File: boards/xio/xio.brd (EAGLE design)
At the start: 170 x 170 mm, 249 parts, among them CN3 J00-0065NL, U2 LAN8742A-CZ, X2 USB-A, Y1 NX3225SA-12.000MHZ-STD-CSR-1, Y2 NX3225SA-12.000MHZ-STD-CSR-1, Y3 NX3225SA-25.000MHZ-STD-CSR-1

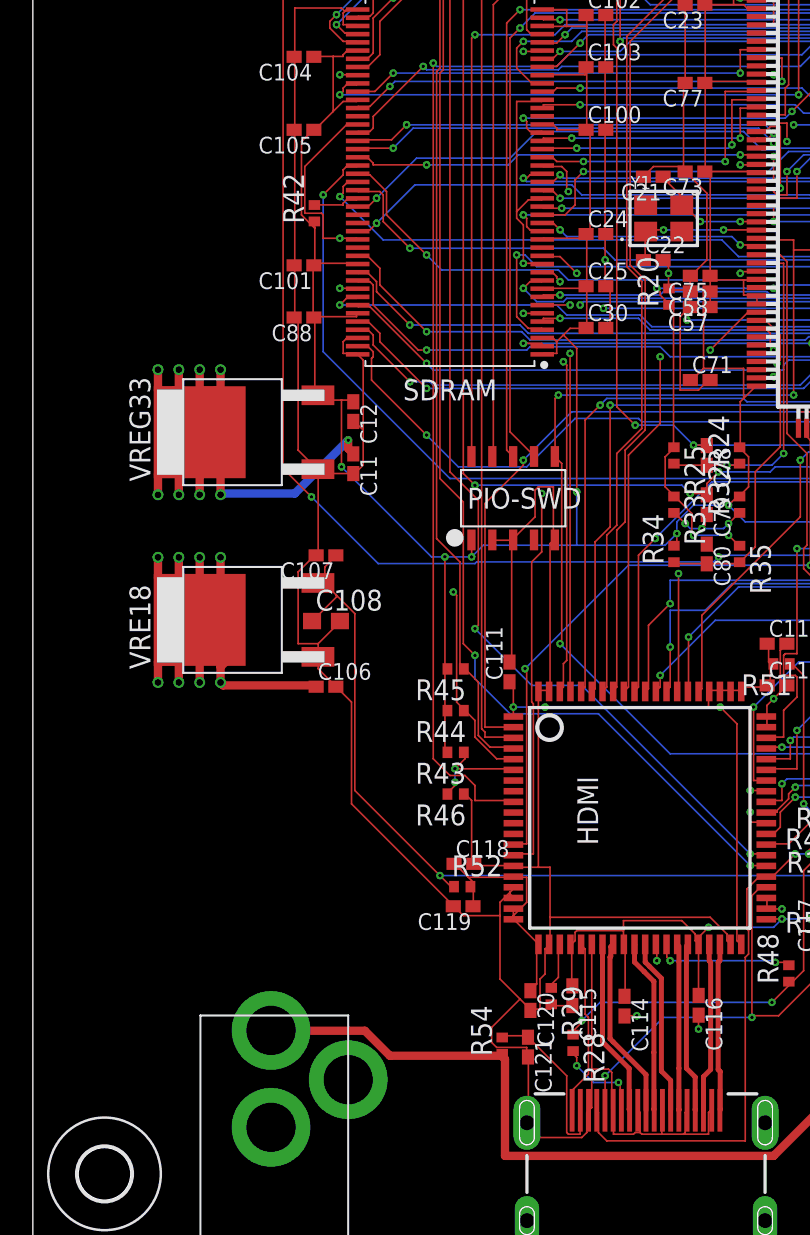
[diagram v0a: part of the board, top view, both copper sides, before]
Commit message: Last minute changes prior to review
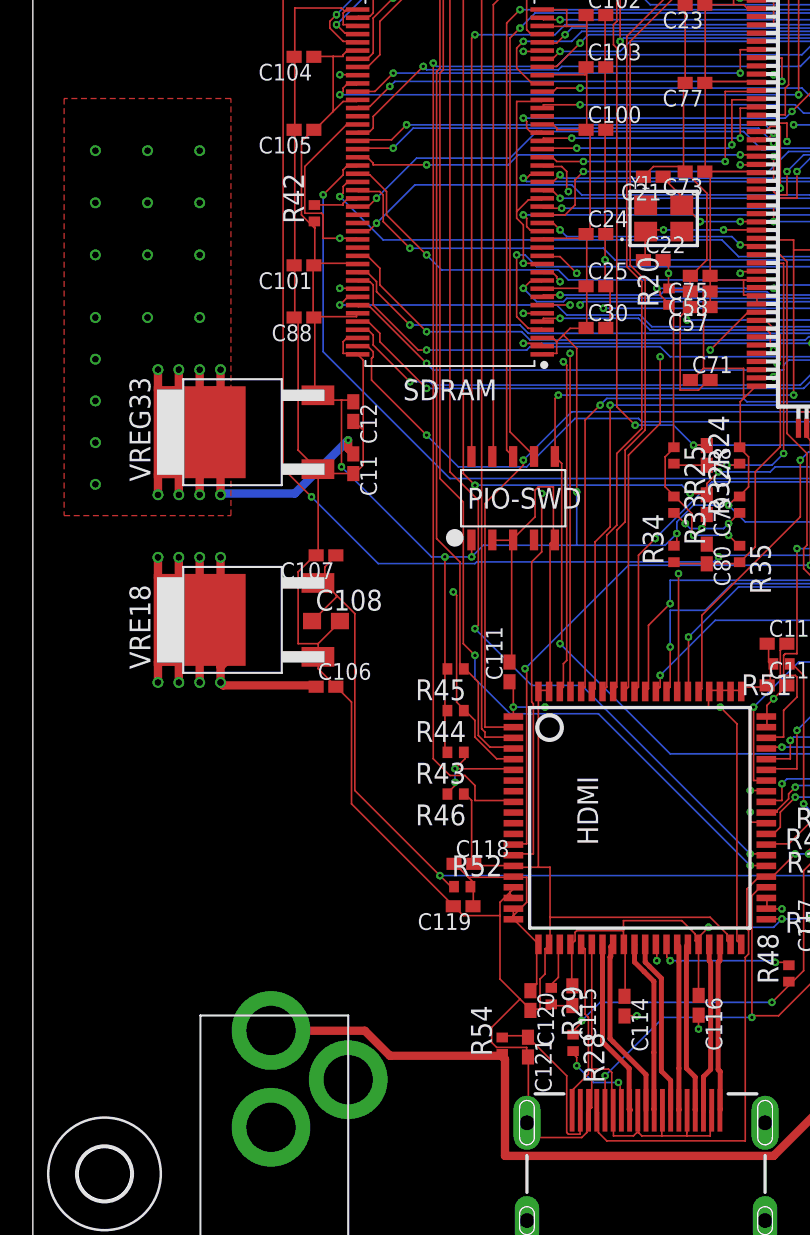
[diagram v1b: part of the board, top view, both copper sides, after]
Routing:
- net +5V: vias 76 -> 92
- added copper zone on layer 1, net +5V
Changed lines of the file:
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@@
 <setting verticaltext="up"/>
 </settings>
-<grid distance="1" unitdist="mil" unit="mil" style="lines" multiple="1" display="yes" altdistance="5" altunitdist="mil" altunit="mil"/>
+<grid distance="0.025" unitdist="inch" unit="inch" style="lines" multiple="1" display="yes" altdistance="5" altunitdist="mil" altunit="mil"/>
 <layers>
 <layer number="1" name="Top" color="4" fill="1" visible="yes" active="yes"/>
@@
 <wire x1="49.5808" y1="84.4296" x2="49.53" y2="84.42" width="0.1016" layer="1"/>
 <wire x1="58.42" y1="84.4296" x2="58.42" y2="84.42" width="0.1016" layer="1"/>
-<wire x1="36.9824" y1="8.7376" x2="36.8808" y2="8.8392" width="0.1016" layer="1"/>
-<wire x1="36.9824" y1="7.5184" x2="36.9824" y2="8.7376" width="0.1016" layer="1"/>
-<wire x1="37.084" y1="7.4168" x2="36.9824" y2="7.5184" width="0.1016" layer="1"/>
-<wire x1="38.3032" y1="7.4168" x2="37.084" y2="7.4168" width="0.1016" layer="1"/>
-<wire x1="38.3032" y1="8.8392" x2="38.3032" y2="7.4168" width="0.1016" layer="1"/>
+<wire x1="36.8808" y1="8.7376" x2="36.8808" y2="8.8392" width="0.1016" layer="1"/>
+<wire x1="36.8808" y1="7.5184" x2="36.8808" y2="8.7376" width="0.1016" layer="1"/>
+<wire x1="37.084" y1="7.3152" x2="36.8808" y2="7.5184" width="0.1016" layer="1"/>
+<wire x1="38.3032" y1="7.3152" x2="37.084" y2="7.3152" width="0.1016" layer="1"/>
+<wire x1="38.3032" y1="8.8392" x2="38.3032" y2="7.3152" width="0.1016" layer="1"/>
 <wire x1="36.8808" y1="8.8392" x2="36.8399" y2="8.8721" width="0.1016" layer="1"/>
 <wire x1="38.3032" y1="8.8392" x2="38.3399" y2="8.8721" width="0.1016" layer="1"/>
-<wire x1="39.7256" y1="8.7376" x2="39.8272" y2="8.8392" width="0.1016" layer="1"/>
-<wire x1="39.7256" y1="7.5184" x2="39.7256" y2="8.7376" width="0.1016" layer="1"/>
-<wire x1="39.624" y1="7.4168" x2="39.7256" y2="7.5184" width="0.1016" layer="1"/>
-<wire x1="38.3032" y1="7.4168" x2="39.624" y2="7.4168" width="0.1016" layer="1"/>
+<wire x1="39.8272" y1="8.7376" x2="39.8272" y2="8.8392" width="0.1016" layer="1"/>
+<wire x1="39.8272" y1="7.5184" x2="39.8272" y2="8.7376" width="0.1016" layer="1"/>
+<wire x1="39.8272" y1="7.3152" x2="39.8272" y2="7.5184" width="0.1016" layer="1"/>
+<wire x1="38.3032" y1="7.3152" x2="39.8272" y2="7.3152" width="0.1016" layer="1"/>
 <wire x1="39.8272" y1="8.8392" x2="39.8399" y2="8.8721" width="0.1016" layer="1"/>
-<wire x1="41.148" y1="8.7376" x2="41.2496" y2="8.8392" width="0.1016" layer="1"/>
-<wire x1="41.148" y1="7.4168" x2="41.148" y2="8.7376" width="0.1016" layer="1"/>
-<wire x1="39.624" y1="7.4168" x2="41.148" y2="7.4168" width="0.1016" layer="1"/>
+<wire x1="41.2496" y1="8.7376" x2="41.2496" y2="8.8392" width="0.1016" layer="1"/>
+<wire x1="41.2496" y1="7.3152" x2="41.2496" y2="8.7376" width="0.1016" layer="1"/>
+<wire x1="39.8272" y1="7.3152" x2="41.2496" y2="7.3152" width="0.1016" layer="1"/>
 <wire x1="41.2496" y1="8.8392" x2="41.3399" y2="8.8721" width="0.1016" layer="1"/>
 <wire x1="34.036" y1="9.0424" x2="34.036" y2="11.3792" width="0.1016" layer="1"/>
@@
 <wire x1="34.036" y1="11.3792" x2="35.052" y2="11.3792" width="0.1016" layer="1"/>
 <wire x1="35.2552" y1="8.9408" x2="35.3399" y2="8.8721" width="0.1016" layer="1"/>
-<wire x1="36.6776" y1="7.5184" x2="36.9824" y2="7.5184" width="0.1016" layer="1"/>
-<wire x1="36.576" y1="7.4168" x2="36.6776" y2="7.5184" width="0.1016" layer="1"/>
-<wire x1="35.3568" y1="7.4168" x2="36.576" y2="7.4168" width="0.1016" layer="1"/>
-<wire x1="35.3568" y1="8.8392" x2="35.3568" y2="7.4168" width="0.1016" layer="1"/>
+<wire x1="36.7792" y1="7.5184" x2="36.8808" y2="7.5184" width="0.1016" layer="1"/>
+<wire x1="36.576" y1="7.3152" x2="36.7792" y2="7.5184" width="0.1016" layer="1"/>
+<wire x1="35.3568" y1="7.3152" x2="36.576" y2="7.3152" width="0.1016" layer="1"/>
+<wire x1="35.3568" y1="8.8392" x2="35.3568" y2="7.3152" width="0.1016" layer="1"/>
 <wire x1="35.3568" y1="8.8392" x2="35.3399" y2="8.8721" width="0.1016" layer="1"/>
 <wire x1="147.1168" y1="30.5816" x2="147.6248" y2="31.0896" width="0.1016" layer="1"/>
@@
 <via x="54.0512" y="25.2984" extent="1-16" drill="0.2"/>
 <via x="19.2024" y="49.6824" extent="1-16" drill="0.2"/>
+<polygon width="0.508" layer="1">
+<vertex x="1.905" y="45.085"/>
+<vertex x="12.065" y="45.085"/>
+<vertex x="12.065" y="70.485"/>
+<vertex x="1.905" y="70.485"/>
+</polygon>
+<via x="10.16" y="57.15" extent="1-16" drill="0.4" locked="yes"/>
+<via x="10.16" y="60.96" extent="1-16" drill="0.4" locked="yes"/>
+<via x="10.16" y="64.135" extent="1-16" drill="0.4" locked="yes"/>
+<via x="10.16" y="67.31" extent="1-16" drill="0.4" locked="yes"/>
+<via x="6.985" y="67.31" extent="1-16" drill="0.4" locked="yes"/>
+<via x="6.985" y="64.135" extent="1-16" drill="0.4" locked="yes"/>
+<via x="6.985" y="60.96" extent="1-16" drill="0.4" locked="yes"/>
+<via x="6.985" y="57.15" extent="1-16" drill="0.4" locked="yes"/>
+<via x="3.81" y="57.15" extent="1-16" drill="0.4" locked="yes"/>
+<via x="3.81" y="60.96" extent="1-16" drill="0.4" locked="yes"/>
+<via x="3.81" y="64.135" extent="1-16" drill="0.4" locked="yes"/>
+<via x="3.81" y="67.31" extent="1-16" drill="0.4" locked="yes"/>
+<via x="3.81" y="46.99" extent="1-16" drill="0.4" locked="yes"/>
+<via x="3.81" y="49.53" extent="1-16" drill="0.4" locked="yes"/>
+<via x="3.81" y="52.07" extent="1-16" drill="0.4" locked="yes"/>
+<via x="3.81" y="54.61" extent="1-16" drill="0.4" locked="yes"/>
 </signal>
 <signal name="!RESET!">
@@
 <wire x1="36.312753125" y1="11.420753125" x2="36.312753125" y2="8.9408" width="0.3048" layer="1" locked="yes"/>
 <wire x1="36.312753125" y1="8.9408" x2="36.312753125" y2="8.899246875" width="0.3048" layer="1" locked="yes"/>
-<wire x1="36.3728" y1="8.9408" x2="36.3399" y2="8.8721" width="0.1016" layer="1"/>
 <wire x1="36.3728" y1="8.9408" x2="36.312753125" y2="8.9408" width="0.1016" layer="1"/>
 <wire x1="36.312753125" y1="11.420753125" x2="34.6899" y2="13.04360625" width="0.3048" layer="1" locked="yes"/>
 <wire x1="34.6899" y1="13.04360625" x2="34.6899" y2="18.9771" width="0.3048" layer="1" locked="yes"/>
+<wire x1="36.3399" y1="8.8721" x2="36.3728" y2="8.8721" width="0.3048" layer="1"/>
+<wire x1="36.3728" y1="8.8721" x2="36.3728" y2="8.9408" width="0.3048" layer="1" locked="yes"/>
 </signal>
 <signal name="TX0_P">
